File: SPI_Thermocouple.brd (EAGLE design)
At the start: 25.1 x 19 mm, 7 parts, among them U1 MAX31855

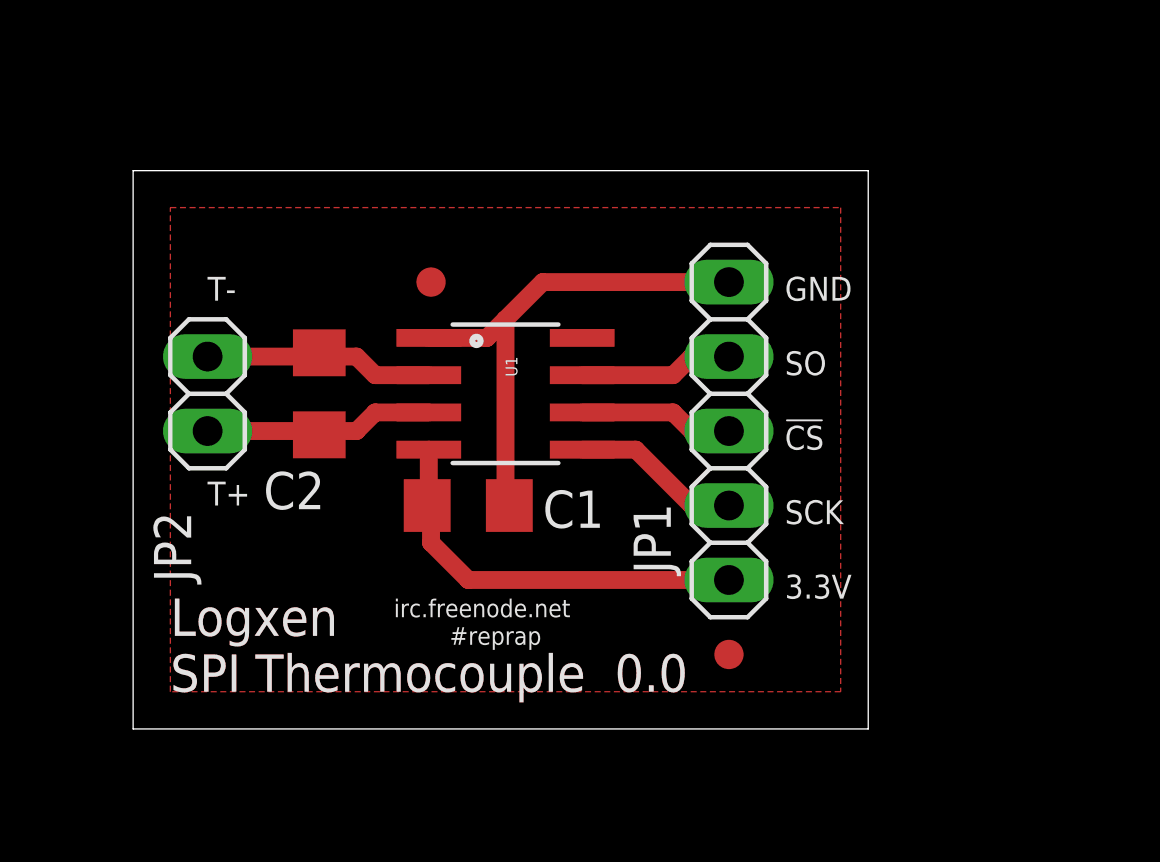
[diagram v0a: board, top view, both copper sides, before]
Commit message: upgrade design to a wing
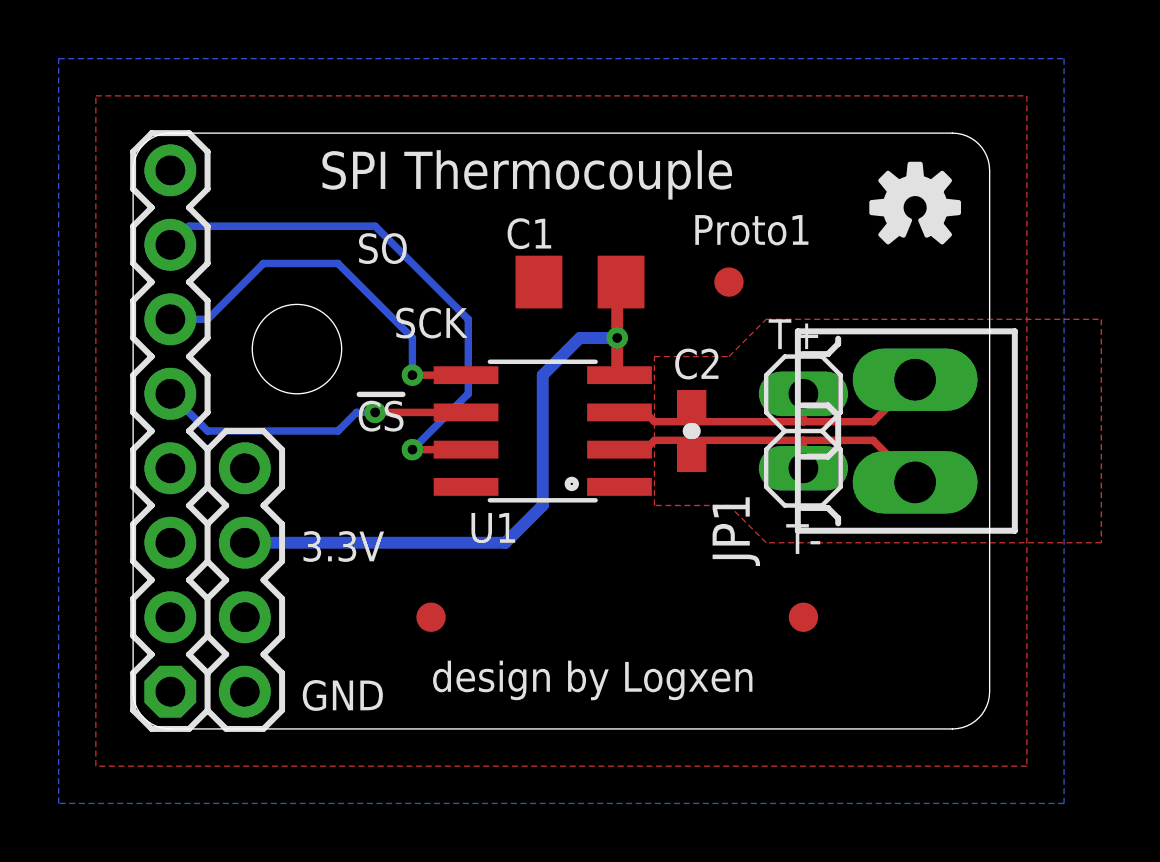
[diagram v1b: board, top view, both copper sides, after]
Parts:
- removed JP2: TC, pinhead:1X02
- removed JP3, JP4: FIDUCIAL1X2, SparkFun:FIDUCIAL-1X2
- added FID1, FID2, FID3: FIDUCIAL1X2, SparkFun:FIDUCIAL-1X2
- added U$1: OSHW-LOGOS, logxen:OSHW-LOGO-S
- added W1: PAPILIO-WING-8BITS, logxen:PAPILIO-WING-8BITS
- added X1: TC, con-weidmueller-sl35:180-2
- C1: device resistor:C1206 -> SparkFun-Passives:1206
- C2: device resistor:C1206 -> SparkFun-Passives:0603-CAP
- JP1: value SPI -> TC; device pinhead:1X05 -> pinhead:1X02
- moved C2 12.8 mm to (19.1, 10.2), turned to 270 degrees
- moved C1 8.52 mm to (15.2, 15.2), turned to 180 degrees
- moved JP1 2.54 mm to (22.9, 10.2)
- moved U1 1.80 mm to (14.0, 10.2), turned to 90 degrees
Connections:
- removed net N$1: C2.1, JP2.1, U1.3
- removed net N$2: C2.2, JP2.2, U1.2
- removed net N$3: JP1.3, U1.6
- removed net N$4: JP1.2, U1.7
- removed net N$5: JP1.4, U1.5
- removed net VCC: C1.1, JP1.5, U1.4
- new net 3.3V: C1.1, U1.4, W1.11
- new net 5V: W1.12
- new net MISO: U1.7, W1.7
- new net N$11: W1.4
- new net N$12: W1.3
- new net N$13: W1.2
- new net N$14: W1.1
- new net N$6: W1.8
- new net SCK: U1.5, W1.6
- new net SSEL: U1.6, W1.5
- new net T+: C2.1, JP1.1, U1.3, X1.1
- new net T-: C2.2, JP1.2, U1.2, X1.2
- net GND: now also W1.9; no longer JP1.1
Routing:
- net 3.3V: track 0.00 -> 21.5 mm, vias 0 -> 1
- net MISO: track 0.00 -> 18.8 mm, vias 0 -> 1
- net GND: track 17.5 -> 0.00 mm
- net VCC: track 14.0 -> 0.00 mm
- net SCK: track 0.00 -> 13.2 mm, vias 0 -> 1
- net T+: track 0.00 -> 12.3 mm
- net T-: track 0.00 -> 12.3 mm
- net SSEL: track 0.00 -> 10.9 mm, vias 0 -> 1
- net N$2: track 7.94 -> 0.00 mm
- net N$1: track 7.94 -> 0.00 mm
- net N$5: track 5.79 -> 0.00 mm
- net N$4: track 5.27 -> 0.00 mm
- net N$3: track 5.27 -> 0.00 mm
- added copper zone on layer 16, net GND
- added copper zone on layer 1, net N$1
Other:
- board size 25.1 x 19 mm -> 29.2 x 20.3 mm
- board text added: "Proto1"
- board text added: "SPI Thermocouple"
- board text added: "design by Logxen"
- board text removed: "#reprap"
- board text removed: "Logxen"
- board text removed: "SPI Thermocouple 0.0"
- board text removed: "irc.freenode.net"
